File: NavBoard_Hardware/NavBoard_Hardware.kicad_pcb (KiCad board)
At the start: 2 copper layers, 61 x 100.1 mm, 43 parts, among them J1 Conn_Coaxial, U3 OKI, U4 OKI, U5 FGPMMOPA6H

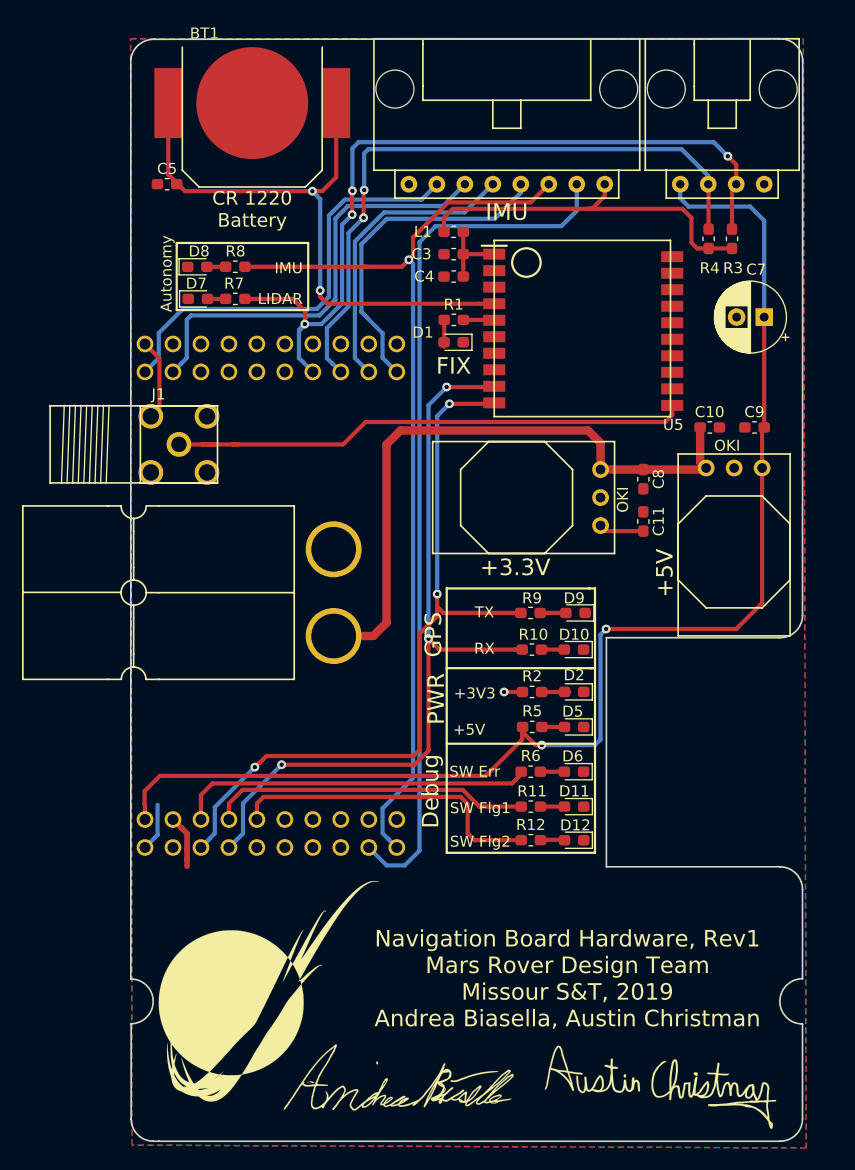
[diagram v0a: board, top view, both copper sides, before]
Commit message: generated step file
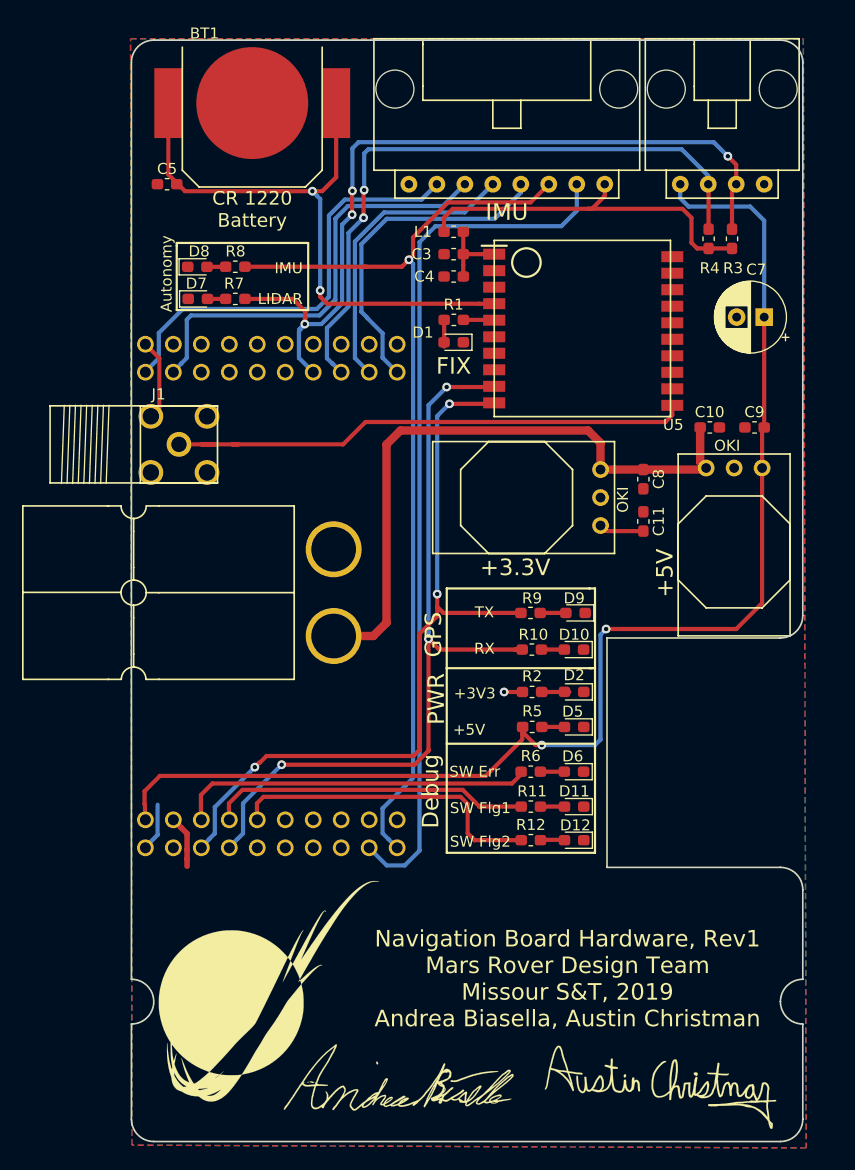
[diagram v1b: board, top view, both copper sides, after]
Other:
- board size 61 x 100.1 mm -> 61 x 100 mm
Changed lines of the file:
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@@
     (47 F.CrtYd user)
     (48 B.Fab user)
-    (49 F.Fab user hide)
+    (49 F.Fab user)
   )
   (setup
-    (last_trace_width 0.762)
+    (last_trace_width 0.25)
     (user_trace_width 0.381)
     (user_trace_width 0.508)
@@
   )
   (module MRDT_Shields:TM4C129E_Launchpad_X9_THT_BOTTOM (layer F.Cu)
-    (at 115.230601 127.024401)
+    (at 115.2652 127.0508)
     (fp_text reference U1 (at 57.404 -0.762 180) (layer F.SilkS) hide
       (effects (font (size 1 1) (thickness 0.15)))
@@
       (xy 1.818986 -2.588809) (xy 1.858404 -2.595946) (xy 1.888683 -2.594105)) (layer F.SilkS) (width 0.01))
   )
+  (gr_line (start 115.2652 137.7188) (end 115.2652 54.483) (layer Edge.Cuts) (width 0.15))
+  (gr_line (start 115.2652 150.4188) (end 115.2652 141.7828) (layer Edge.Cuts) (width 0.15))
+  (gr_line (start 174.1932 152.4508) (end 117.2972 152.4508) (layer Edge.Cuts) (width 0.15))
+  (gr_line (start 176.2252 141.7828) (end 176.2252 150.4188) (layer Edge.Cuts) (width 0.15))
+  (gr_line (start 176.2252 129.5908) (end 176.2252 137.7188) (layer Edge.Cuts) (width 0.15))
+  (gr_line (start 158.4452 127.5588) (end 174.1932 127.5588) (layer Edge.Cuts) (width 0.15))
+  (gr_line (start 158.4452 106.7308) (end 158.4452 127.5588) (layer Edge.Cuts) (width 0.15))
+  (gr_line (start 174.1932 106.7308) (end 158.4452 106.7308) (layer Edge.Cuts) (width 0.15))
+  (gr_line (start 176.2252 54.483) (end 176.2252 104.6988) (layer Edge.Cuts) (width 0.15))
+  (gr_line (start 117.2972 52.451) (end 174.1932 52.451) (layer Edge.Cuts) (width 0.15))
+  (gr_arc (start 117.2972 54.483) (end 117.2972 52.451) (angle -90) (layer Edge.Cuts) (width 0.15))
+  (gr_arc (start 174.1932 54.483) (end 176.2252 54.483) (angle -90) (layer Edge.Cuts) (width 0.15))
+  (gr_arc (start 174.1932 104.6988) (end 174.1932 106.7308) (angle -90) (layer Edge.Cuts) (width 0.15))
+  (gr_arc (start 174.1932 129.5908) (end 176.2252 129.5908) (angle -90) (layer Edge.Cuts) (width 0.15))
+  (gr_arc (start 176.2252 139.7508) (end 176.2252 137.7188) (angle -90) (layer Edge.Cuts) (width 0.15))
+  (gr_arc (start 176.2252 139.7508) (end 174.1932 139.7508) (angle -90) (layer Edge.Cuts) (width 0.15))
+  (gr_arc (start 174.1932 150.4188) (end 174.1932 152.4508) (angle -90) (layer Edge.Cuts) (width 0.15))
+  (gr_arc (start 117.2972 150.4188) (end 115.2652 150.4188) (angle -90) (layer Edge.Cuts) (width 0.15))
+  (gr_arc (start 115.2652 139.7508) (end 115.2652 141.7828) (angle -180) (layer Edge.Cuts) (width 0.15))
   (gr_text "FIX\n" (at 144.526 82.042) (layer F.SilkS)
     (effects (font (size 1.5 1.5) (thickness 0.3)))
@@
   (gr_circle (center 151.13 72.644) (end 152.4 72.898) (layer F.SilkS) (width 0.2))
   (gr_line (start 147.066 71.12) (end 149.352 71.12) (layer F.SilkS) (width 0.2))
-  (gr_arc (start 117.2972 54.478921) (end 117.399059 52.3748) (angle -83.65369847) (layer Edge.Cuts) (width 0.15))
-  (gr_arc (start 174.1805 54.356) (end 176.2125 54.356) (angle -93.93289733) (layer Edge.Cuts) (width 0.15))
   (gr_text "GPS\n\n" (at 143.8965 106.426 90) (layer F.SilkS)
     (effects (font (size 1.5 1.5) (thickness 0.3)))
@@
     (effects (font (size 1.5 1.5) (thickness 0.3)))
   )
-  (gr_line (start 115.2398 150.3934) (end 115.2398 141.7574) (layer Edge.Cuts) (width 0.15))
-  (gr_line (start 117.7544 152.4254) (end 117.2718 152.4254) (layer Edge.Cuts) (width 0.15))
-  (gr_arc (start 117.2718 150.3934) (end 115.2398 150.3934) (angle -90) (layer Edge.Cuts) (width 0.15))
-  (gr_arc (start 115.2144 139.7254) (end 115.2144 141.7574) (angle -180) (layer Edge.Cuts) (width 0.15))
-  (gr_line (start 115.2144 54.1528) (end 115.2144 137.668) (layer Edge.Cuts) (width 0.15))
-  (gr_line (start 174.0535 52.324) (end 117.3988 52.3748) (layer Edge.Cuts) (width 0.15))
-  (gr_line (start 176.1998 104.6734) (end 176.2125 54.356) (layer Edge.Cuts) (width 0.15))
-  (gr_arc (start 174.1678 104.6734) (end 174.142401 106.705399) (angle -90.71615995) (layer Edge.Cuts) (width 0.15))
-  (gr_line (start 158.3944 106.7054) (end 174.1424 106.7054) (layer Edge.Cuts) (width 0.15))
-  (gr_line (start 158.3944 127.508) (end 158.3944 106.7054) (layer Edge.Cuts) (width 0.15))
-  (gr_line (start 174.1678 127.508) (end 158.3944 127.508) (layer Edge.Cuts) (width 0.15))
-  (gr_arc (start 174.1424 129.5654) (end 176.1998 129.5654) (angle -90) (layer Edge.Cuts) (width 0.15))
-  (gr_line (start 176.1998 137.668) (end 176.1998 129.5654) (layer Edge.Cuts) (width 0.15))
-  (gr_arc (start 176.1998 139.7254) (end 176.1998 137.668) (angle -180) (layer Edge.Cuts) (width 0.15))
-  (gr_line (start 176.1998 150.3934) (end 176.1998 141.7828) (layer Edge.Cuts) (width 0.15))
-  (gr_arc (start 174.1678 150.3934) (end 174.1678 152.4254) (angle -90) (layer Edge.Cuts) (width 0.15))
-  (gr_line (start 117.7798 152.4254) (end 174.1678 152.4254) (layer Edge.Cuts) (width 0.15))
   (segment (start 119.8006 123.9744) (end 119.8088 123.9744) (width 0.508) (layer F.Cu) (net 1))
   (segment (start 119.040601 123.214401) (end 119.8006 123.9744) (width 0.508) (layer F.Cu) (net 1))
@@
   (segment (start 117.651102 124.6039) (end 117.651102 121.870898) (width 0.381) (layer B.Cu) (net 7))
   (segment (start 116.500601 125.754401) (end 117.651102 124.6039) (width 0.381) (layer B.Cu) (net 7))
-  (segment (start 143.665 80.25) (end 143.651 80.264) (width 0.381) (layer F.Cu) (net 8))
-  (segment (start 143.665 78.232) (end 143.665 80.25) (width 0.381) (layer F.Cu) (net 8))
-  (segment (start 155.027921 111.633) (end 155.036421 111.6245) (width 0.381) (layer F.Cu) (net 9))
-  (segment (start 154.57 111.633) (end 154.5785 111.6245) (width 0.381) (layer F.Cu) (net 9))
-  (segment (start 152.5185 111.633) (end 154.062 111.633) (width 0.381) (layer F.Cu) (net 9))
-  (segment (start 148.178 77.851) (end 148.209 77.882) (width 0.381) (layer F.Cu) (net 10))
-  (segment (start 145.415 77.851) (end 148.178 77.851) (width 0.381) (layer F.Cu) (net 10))
   (segment (start 169.799 71.363388) (end 167.673606 71.363388) (width 0.381) (layer F.Cu) (net 7))
   (segment (start 156.718 67.76401) (end 144.45299 67.76401) (width 0.381) (layer F.Cu) (net 7))
@@
   (segment (start 165.30001 67.76401) (end 166.116 68.58) (width 0.381) (layer F.Cu) (net 7))
   (segment (start 156.718 67.76401) (end 165.30001 67.76401) (width 0.381) (layer F.Cu) (net 7))
+  (segment (start 143.665 80.25) (end 143.651 80.264) (width 0.381) (layer F.Cu) (net 8))
+  (segment (start 143.665 78.232) (end 143.665 80.25) (width 0.381) (layer F.Cu) (net 8))
+  (segment (start 155.027921 111.633) (end 155.036421 111.6245) (width 0.381) (layer F.Cu) (net 9))
+  (segment (start 154.57 111.633) (end 154.5785 111.6245) (width 0.381) (layer F.Cu) (net 9))
+  (segment (start 152.5185 111.633) (end 154.062 111.633) (width 0.381) (layer F.Cu) (net 9))
+  (segment (start 148.178 77.851) (end 148.209 77.882) (width 0.381) (layer F.Cu) (net 10))
+  (segment (start 145.415 77.851) (end 148.178 77.851) (width 0.381) (layer F.Cu) (net 10))
   (segment (start 116.500601 121.878399) (end 116.500601 123.214401) (width 0.381) (layer F.Cu) (net 11))
   (segment (start 116.459 121.836798) (end 116.500601 121.878399) (width 0.381) (layer F.Cu) (net 11))
